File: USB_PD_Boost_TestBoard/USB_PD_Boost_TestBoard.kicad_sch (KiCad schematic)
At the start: 7 parts, among them J1 USB_C_Receptacle_USB2.0_16P

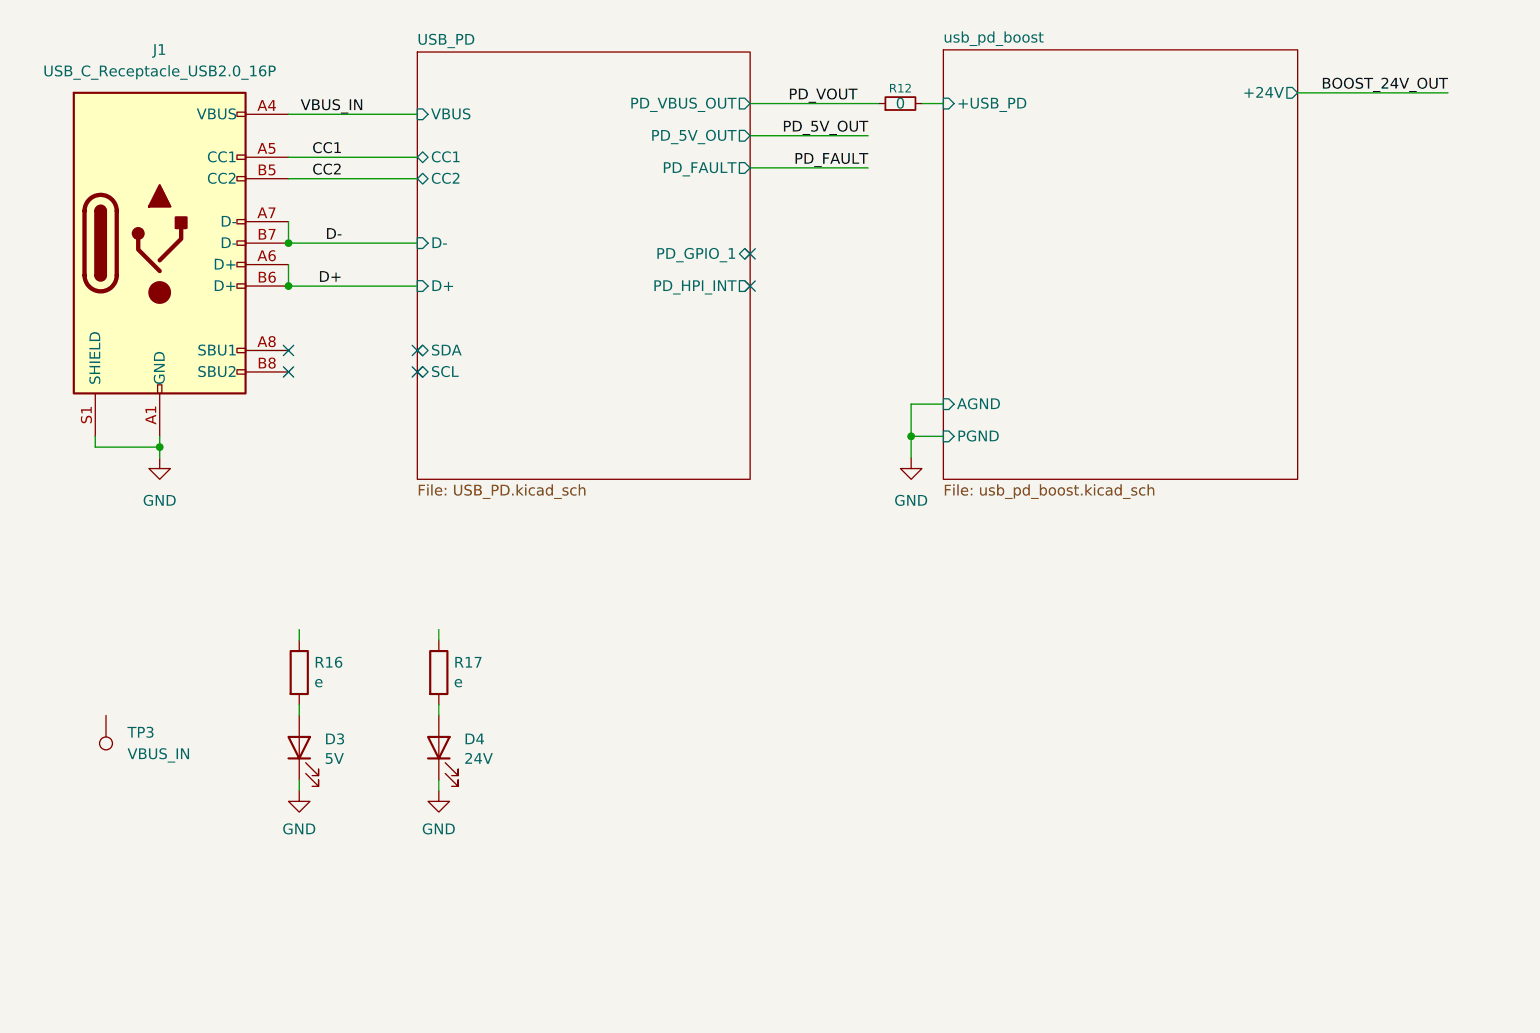
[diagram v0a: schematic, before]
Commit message: some stuff
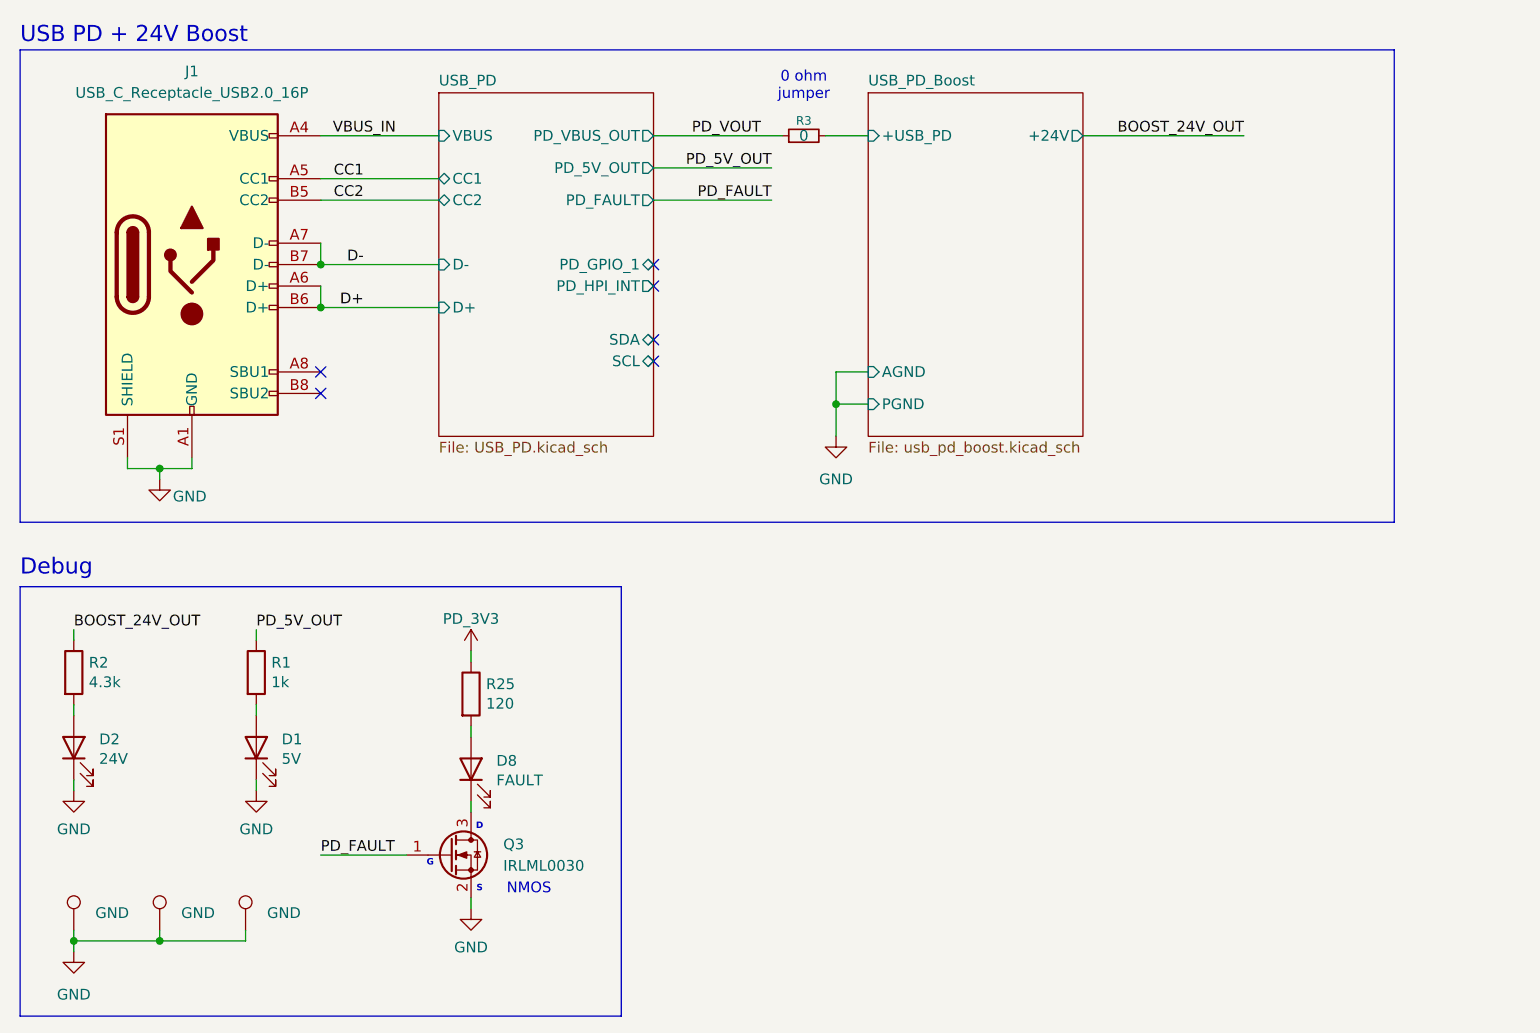
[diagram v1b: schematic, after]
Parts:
- removed TP3: VBUS_IN, TestPoint:TestPoint_Pad_1.0x1.0mm, symbol Connector:TestPoint
- added D8: FAULT, LED_SMD:LED_0603_1608Metric_Pad1.05x0.95mm_HandSolder, symbol Device:LED
- added Q3: IRLML0030, Package_TO_SOT_SMD:SOT-23, symbol Transistor_FET:IRLML0030
- added R25: 120, Resistor_SMD:R_0603_1608Metric_Pad0.98x0.95mm_HandSolder, symbol Device:R
- added TP1, TP10, TP9: GND, TestPoint:TestPoint_Pad_1.0x1.0mm, symbol Connector:TestPoint
- R1: renamed from R16; value e -> 1k
- R2: renamed from R17; value e -> 4.3k
- renumbered D3 to D1, D4 to D2, R12 to R3
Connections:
- net BOOST_24V_OUT: now also R2.1
- net GND: now also Q3.2 (S), TP1.1, TP10.1, TP9.1
- net PD_5V_OUT: now also R1.1
- net PD_FAULT: now also Q3.1 (G)
- new net: D8.1 (K), Q3.3 (D)
- new net: D8.2 (A), R25.2
- new net PD_3V3: R25.1
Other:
- sheet usb_pd_boost renamed USB_PD_Boost
- note added: "0 ohm jumper"
- note added: "D"
- note added: "Debug"
- note added: "G"
- note added: "NMOS"
- note added: "S"
- note added: "USB PD + 24V Boost"
- moved on the sheet: D1, D2, J1, R1, R2, R3

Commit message: idk
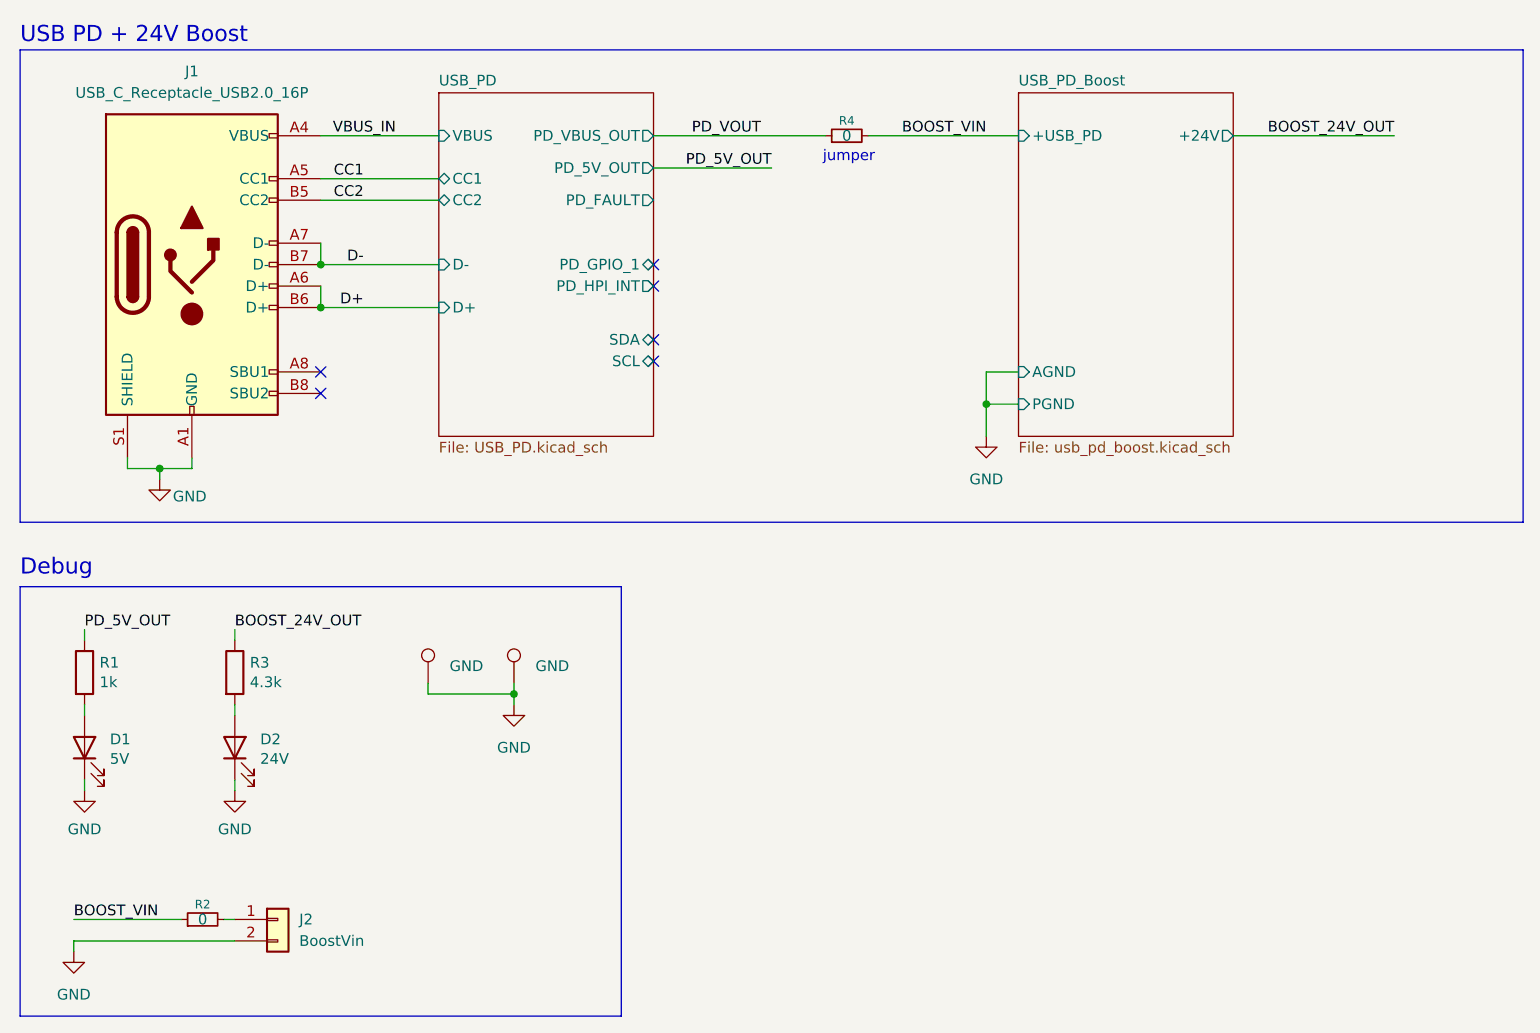
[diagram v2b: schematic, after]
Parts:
- removed D8: FAULT, LED_SMD:LED_0603_1608Metric_Pad1.05x0.95mm_HandSolder, symbol Device:LED
- removed Q3: IRLML0030, Package_TO_SOT_SMD:SOT-23, symbol Transistor_FET:IRLML0030
- removed R25: 120, Resistor_SMD:R_0603_1608Metric_Pad0.98x0.95mm_HandSolder, symbol Device:R
- removed TP1: GND, TestPoint:TestPoint_Pad_1.0x1.0mm, symbol Connector:TestPoint
- added J2: BoostVin, symbol Connector_Generic:Conn_01x02
- added R2: 0, symbol Device:R_Small
- renumbered R2 to R3, R3 to R4, TP9 to TP1, TP10 to TP2
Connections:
- net GND: now also J2.2 (Pin_2)
- net USB_PD_Boost/+USB_PD renamed BOOST_VIN
- net BOOST_VIN: now also R2.1
- new net: J2.1 (Pin_1), R2.2
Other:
- note added: "jumper"
- note removed: "0 ohm jumper"
- note removed: "D"
- note removed: "G"
- note removed: "NMOS"
- note removed: "S"
- moved on the sheet: D1, D2, R1, R3, R4
